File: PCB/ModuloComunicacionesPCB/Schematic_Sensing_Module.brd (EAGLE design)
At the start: 160 x 100 mm, 73 parts, among them J1 TERMINAL-TB3, J2 TERMINAL-TB3, J3 TERMINAL-TB3, J4 TERMINAL-TB3, Q1 CSM-7X-DU, Q2 MMBT2222A, SW2 1825910-6, U1 ATMEGA328P-PU, U2 LP38692MP-5.0, U3 MCP1501T-18E/SN, U4 ACS723LLCTR-05AB-T, U5 OPA320AIDBVR

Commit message: avances en placing de la pcb del transmisor
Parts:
- removed BAT_PIN: (no value), pinhead:1X02
- removed C24: (no value), rcl:C0805
- removed FTDI_PIN: (no value), pinhead:1X04
- removed J1, J2, J3, J4: TERMINAL-TB3, TERMINAL-TB001:TERMINAL-TB3
- removed Q2: MMBT2222A, MMBT2222A:SOT23
- removed R15, R16, R17, R3, R4, R5: 0.1, rcl:R1206
- removed U$2, U$7: REF3450, SOT95P280X145-6N:SOT95P280X145-6N
- removed U$3: MCP6002-E/MS, MCP6002-E_MS:SOP65P490X110-8N
- removed U$6: TERMINAL-TB2, TERMINAL-TB001:TERMINAL-TB2
- removed U2: LP38692MP-5.0, LP38692MP-5.0:SOT150P696X180-5N
- removed U4: ACS723LLCTR-05AB-T, ACS723LLCTR-05AB-T:SOIC127P600X175-8N
- removed U5: OPA320AIDBVR, OPA320AIDBVR:SOT95P280X145-5N
- added 2N2222: MMBT2222A, MMBT2222A:SOT23
- added ACS723: ACS723LLCTR-05AB-T, ACS723LLCTR-05AB-T:SOIC127P600X175-8N
- added C29, C30, C31, C32: 0.1uF, rcl:C1206
- added C33: 1nF, rcl:C1206
- added C34, C35: 2.2uF, rcl:C1206
- added IACT: (no value), TERMINAL-TB001:TERMINAL-TB2
- added JP1: (no value), pinhead:1X04/90
- added LP38692: LP38692MP-5.0, LP38692MP-5.0:SOT150P696X180-5N
- added MCP6002: MCP6002-E/MS, MCP6002-E_MS:SOP65P490X110-8N
- added OPA320: OPA320AIDBVR, OPA320AIDBVR:SOT95P280X145-5N
- added R3450, REF3450: REF3450, SOT95P280X145-6N:SOT95P280X145-6N
- added TS1, TS2, WS1, WS2: (no value), TERMINAL-TB001:TERMINAL-TB3
- C11, C12: value 22p -> 22pF; device rcl:C1206 -> rcl:C0805
- C14, C15, C20, C21: value 100n -> 100nF
- C17: value 8.2pF -> 18pF
- C2, C3: value 1uF -> cambiar por los de 10uF ceramicos de didacticas
- C22: value 0.1u -> 0.1uF
- C25, C26, C27, C28: value 0.1nF -> 0.1uF
- U$4: value INA219_BB -> INABB; device INA219_BB:INA219_BB -> INA219BB:INA219-MODULE
- moved C27 315.3 mm to (98.1, 114.0)
- moved C28 309.0 mm to (80.7, 116.0)
- moved C22 235.1 mm to (151.1, 114.0)
- moved C25 210.0 mm to (60.2, 23.8), turned to 180 degrees
- moved U$8 208.7 mm to (83.3, 59.1), turned to 270 degrees
- moved R19 205.8 mm to (60.1, 18.4), turned to 180 degrees
- moved LED4 199.4 mm to (115.7, 74.0), turned to 90 degrees
- moved C26 196.9 mm to (46.2, 17.6), turned to 270 degrees
- moved LED3 195.6 mm to (116.1, 66.9), turned to 270 degrees
- moved R1 192.7 mm to (90.5, 38.5), turned to 180 degrees
- moved R12 191.1 mm to (98.1, 106.3)
- moved R7 189.3 mm to (107.7, 67.0), turned to 180 degrees
- moved SW2 187.5 mm to (115.8, 57.7), turned to 90 degrees
- moved R18 186.2 mm to (41.4, 17.6), turned to 270 degrees
- moved C23 170.4 mm to (66.0, 38.5)
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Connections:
- removed net +5V: U$1.IN+
- removed net A0: U1.23
- removed net A1: U1.24
- removed net A2: U1.25
- removed net A3: U1.26
- removed net N$1: R3.2, U$2.1
- removed net N$10: U$6.1, U4.1, U4.2
- removed net N$11: U$6.2, U4.3, U4.4
- removed net N$12: R11.2, U4.7
- removed net N$13: C9.1, R12.2, U5.3
- removed net N$15: C10.1, R13.1, U5.1, U5.4
- removed net N$18: R16.2, U$7.6
- removed net N$19: R17.2, U$7.5
- removed net N$20: R15.2, U$7.1
- removed net N$24: C25.1, R19.1, U$3.3
- removed net N$25: C26.1, R18.1, U$3.5
- removed net N$5: R4.2, U$2.6
- removed net N$6: R5.2, U$2.5
- removed net N$8: R10.1, U4.6
- removed net VOUT-: U$1.VOUT-
- new net BWSEL: ACS723.6, R10.1
- new net IP+: ACS723.1, ACS723.2, IACT.1
- new net IP-: ACS723.3, ACS723.4, IACT.2
- new net VIN+: C9.1, OPA320.3, R12.2
- new net VIN-: C10.1, OPA320.1, OPA320.4, R13.1
- new net VO: ACS723.7, C33.1, R11.2
- net B+INA: now also U$4.6
- net B-INA: now also U$4.5; no longer BAT_PIN.1
- net BATL: now also U1.13; no longer U1.11
- net DATAT1: now also TS1.2, U1.14; no longer J3.2
- net DATAT2: now also TS2.2, U1.15; no longer J4.2
- net DATAW1: now also C25.1, MCP6002.3, R19.1, WS1.3; no longer J1.3
- net DATAW2: now also C26.1, MCP6002.5, R18.1, WS2.3; no longer J2.3
- net DTR: now also JP1.4; no longer FTDI_PIN.4
- net GND: now also ACS723.5, C29.2, C30.2, C31.2, C32.2, C33.2, C34.1, C35.2, JP1.1, LP38692.5, MCP6002.4, OPA320.2, R3450.1, R3450.2, REF3450.1, REF3450.2, TS1.3, TS2.3, U$1.VOUT-, U$4.2, U$8.DIO0, U$8.DIO1, U$8.DIO2, U$8.DIO3, U$8.DIO4, U1.25, U1.26, U1.6, WS1.1, WS2.1; no longer BAT_PIN.2, C24.2, FTDI_PIN.1, J1.1, J2.1, J3.3, J4.3, R15.1, R3.1, U$2.2, U$3.4, U$7.2, U2.5, U4.5, U5.2
- net N$2: now also 2N2222.1; no longer Q2.1
- net OSC+: now also C12.1; no longer C11.1
- net OSC-: now also C11.1; no longer C12.1
- net RX0: now also JP1.3; no longer FTDI_PIN.3
- net RX1: now also U$8.TX
- net SCL: now also U$4.3
- net SDA: now also U$4.4
- net TX0: now also JP1.2; no longer FTDI_PIN.2
- net TX1: now also U$8.RX
- net VACS: now also ACS723.8, REF3450.5, REF3450.6; no longer R16.1, R17.1, U4.8
- net VDD33: now also C29.1, U$4.1; no longer C17.1, C24.1
- net VLP5: now also C30.1, C31.1, C32.1, C34.2, LP38692.3, MCP6002.8, TS1.1, TS2.1, U1.21, WS1.2, WS2.2; no longer J1.2, J2.2, J3.1, J4.1, U$3.8, U2.3
- net VOREG: now also 2N2222.2, R3450.3, R3450.4, REF3450.3, REF3450.4; no longer Q2.2, U$2.3, U$2.4, U$7.3, U$7.4
- net VOUT+: now also C17.1, C35.1
- net VOW1: now also MCP6002.1, MCP6002.2, U1.23; no longer U$3.1, U$3.2
- net VOW2: now also MCP6002.6, MCP6002.7, U1.24; no longer U$3.6, U$3.7
- net VREF5: now also OPA320.5, R3450.5, R3450.6; no longer R4.1, R5.1, U5.5
- net VSUPPLY: now also 2N2222.3, LP38692.1, LP38692.4; no longer Q2.3, U2.1, U2.4

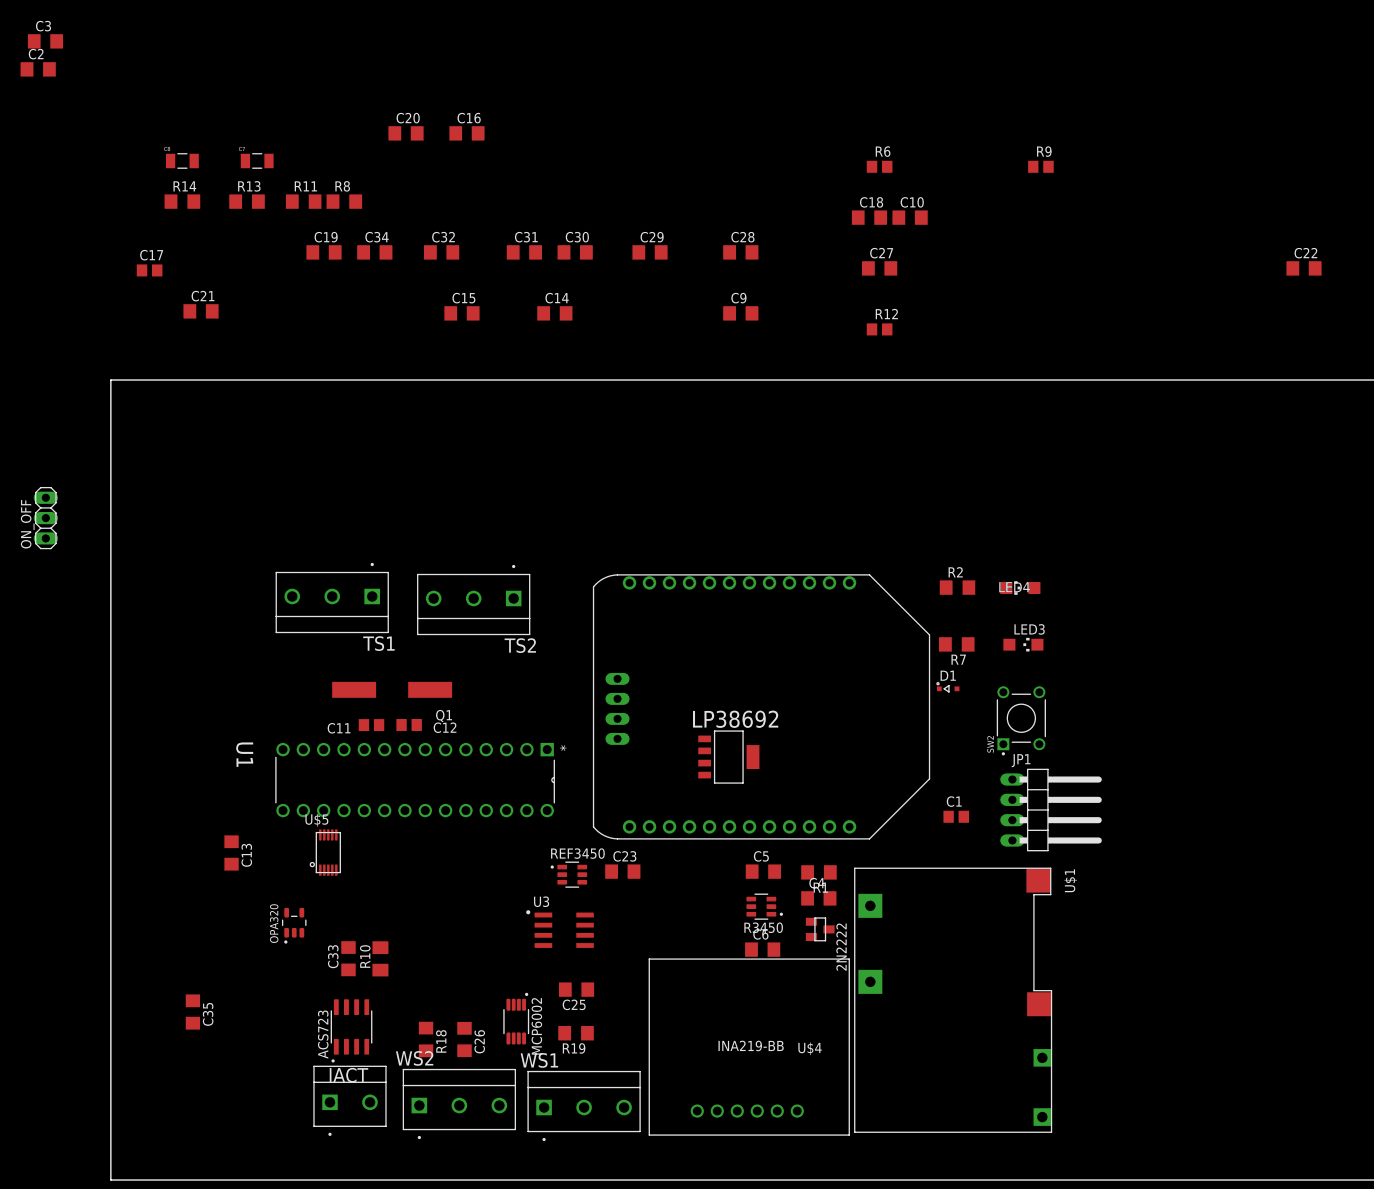
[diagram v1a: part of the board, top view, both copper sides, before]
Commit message: placing almost done
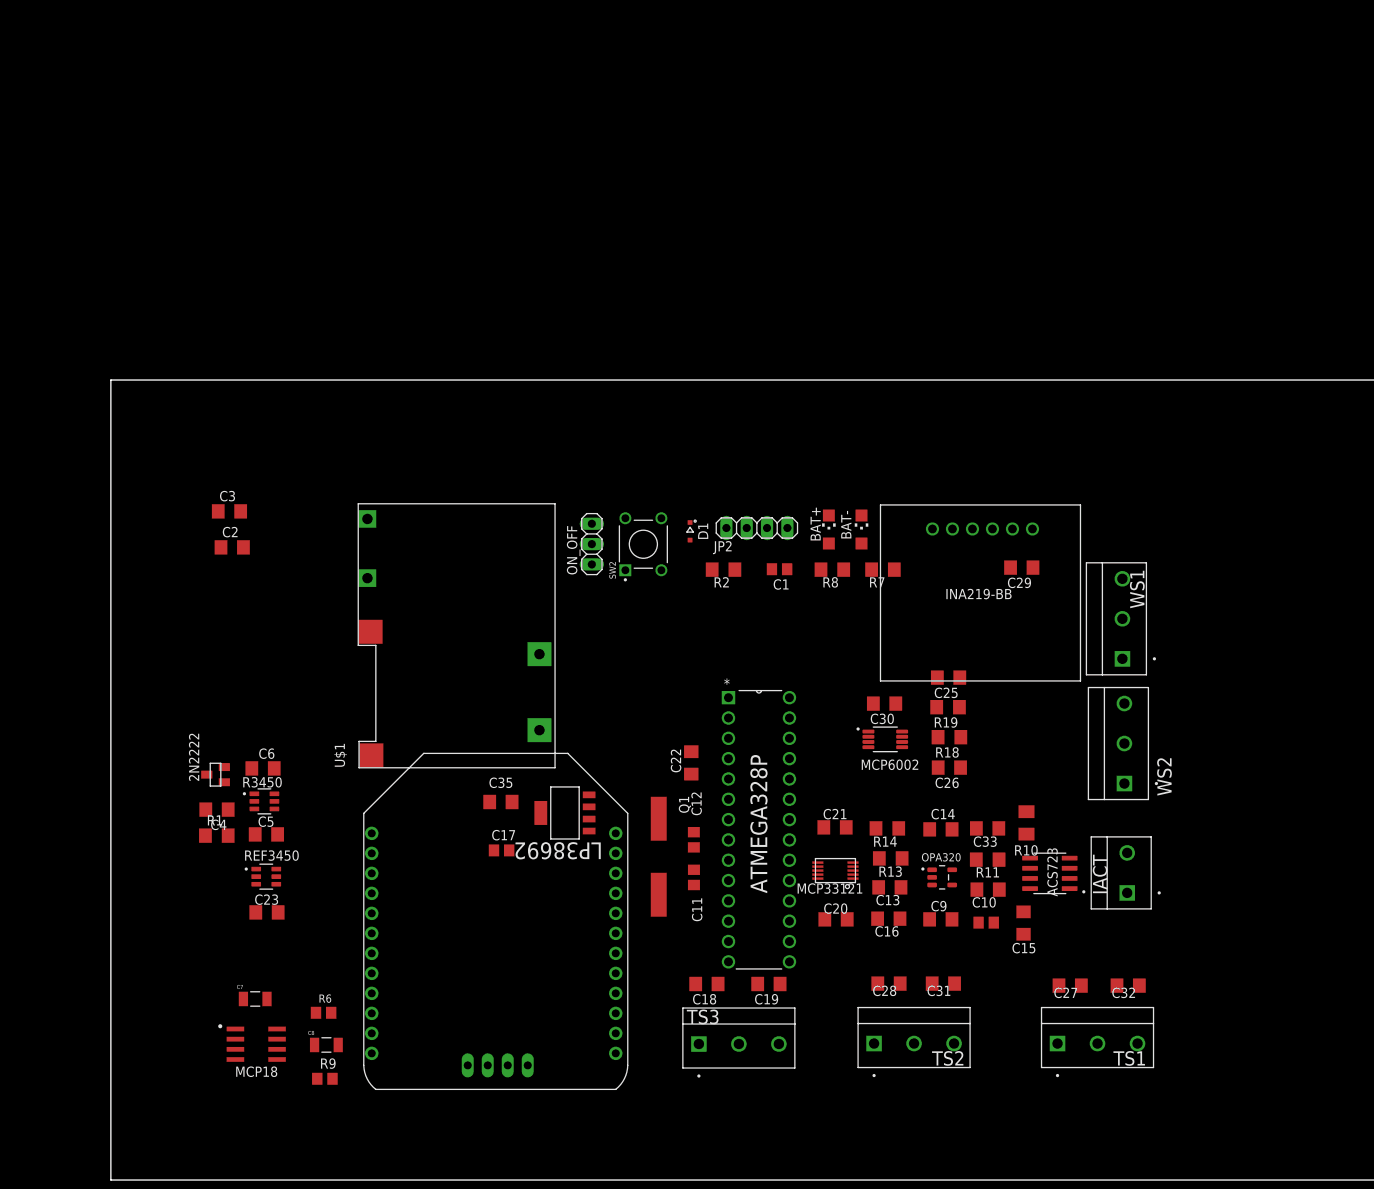
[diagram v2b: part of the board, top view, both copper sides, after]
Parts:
- removed C34: 2.2uF, rcl:C1206
- removed JP1: (no value), pinhead:1X04/90
- removed LED3, LED4: (no value), led:CHIPLED_1206
- removed U$4: INABB, INA219BB:INA219-MODULE
- removed U$5: MCP33121, mcp33121:MSOP10
- removed U1: ATMEGA328P-PU, Atmel_By_element14_Batch_1-00:DIP254P762X457-28
- removed U3: MCP1501T-18E/SN, MCP1501T-18E_SN:SOIC127P600X175-8N
- added ATMEGA328P: ATMEGA328P-PU, Atmel_By_element14_Batch_1-00:DIP254P762X457-28
- added BAT+, BAT-: (no value), led:CHIPLED_1206
- added INA219: INABB, INA219BB:INA219-MODULE
- added JP2: (no value), pinhead:1X04
- added MCP18: MCP1501T-18E/SN, MCP1501T-18E_SN:SOIC127P600X175-8N
- added MCP33121: MCP33121, mcp33121:MSOP10
- added TS3: (no value), TERMINAL-TB001:TERMINAL-TB3
- C18: value 1uF -> 0.1uF
- C19: value 10uF -> 0.1uF
- moved R9 144.9 mm to (28.8, 12.7)
- moved R6 126.5 mm to (28.6, 20.9)
- moved C32 125.6 mm to (129.2, 24.3), turned to 180 degrees
- moved R11 118.6 mm to (111.6, 40.0)
- moved R14 117.9 mm to (99.1, 44.0), turned to 180 degrees
- moved R13 115.0 mm to (99.5, 40.2), turned to 180 degrees
- moved C20 112.0 mm to (92.6, 32.6), turned to 180 degrees
- moved C8 112.0 mm to (28.9, 16.9)
- moved C16 111.4 mm to (99.2, 32.7)
- moved C19 107.0 mm to (84.2, 24.5), turned to 180 degrees
- moved C31 105.3 mm to (106.1, 24.6), turned to 180 degrees
- moved C7 104.8 mm to (20.0, 22.6)
- moved C15 103.6 mm to (116.1, 32.1), turned to 270 degrees
- moved C21 102.2 mm to (92.5, 44.1)
- moved IACT 101.3 mm to (129.0, 38.4), turned to 90 degrees
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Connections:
- removed net N$16: C13.2, R13.2, U$5.3
- removed net N$17: C13.1, R14.2, U$5.4
- removed net N$7: R6.2, R9.2, U3.7, U3.8
- new net DATAT3: ATMEGA328P.13, C18.1, TS3.2
- new net IN+: C13.2, MCP33121.3, R13.2
- new net IN-: C13.1, MCP33121.4, R14.2
- new net VOMCP18: MCP18.7, MCP18.8, R6.2, R9.2
- net AMISO: now also ATMEGA328P.18, MCP33121.7; no longer U$5.7, U1.18
- net AMOSI: now also ATMEGA328P.17, MCP33121.9; no longer U$5.9, U1.17
- net ASCK: now also ATMEGA328P.19, MCP33121.8; no longer U$5.8, U1.19
- net ASS: now also ATMEGA328P.16, MCP33121.6; no longer U$5.6, U1.16
- net B+INA: now also INA219.6; no longer U$4.6
- net B-INA: now also INA219.5; no longer U$4.5
- net BATH: now also ATMEGA328P.11; no longer U1.12
- net BATL: now also ATMEGA328P.12; no longer U1.13
- net DATAT1: now also ATMEGA328P.14; no longer U1.14
- net DATAT2: now also ATMEGA328P.15; no longer U1.15
- net DTR: now also JP2.4; no longer JP1.4
- net GND: now also ATMEGA328P.22, ATMEGA328P.25, ATMEGA328P.26, ATMEGA328P.6, ATMEGA328P.8, BAT+.C, BAT-.C, C19.2, INA219.2, JP2.1, MCP18.2, MCP18.4, MCP18.5, MCP18.6, MCP33121.5, TS1.1, TS2.1, TS3.1; no longer C19.1, C34.1, JP1.1, LED3.C, LED4.C, TS1.3, TS2.3, U$4.2, U$5.5, U1.22, U1.25, U1.26, U1.6, U1.8, U3.2, U3.4, U3.5, U3.6
- net N$3: now also BAT-.A; no longer LED3.A
- net N$4: now also BAT+.A; no longer LED4.A
- net OSC+: now also ATMEGA328P.9; no longer U1.9
- net OSC-: now also ATMEGA328P.10; no longer U1.10
- net RST: now also ATMEGA328P.1; no longer U1.1
- net RX0: now also ATMEGA328P.2, JP2.3; no longer JP1.3, U1.2
- net RX1: now also ATMEGA328P.4; no longer U1.4
- net SCL: now also ATMEGA328P.28, INA219.3; no longer U$4.3, U1.28
- net SDA: now also ATMEGA328P.27, INA219.4; no longer U$4.4, U1.27
- net TX0: now also ATMEGA328P.3, JP2.2; no longer JP1.2, U1.3
- net TX1: now also ATMEGA328P.5; no longer U1.5
- net VDD33: now also INA219.1; no longer U$4.1
- net VLP5: now also ATMEGA328P.20, ATMEGA328P.21, ATMEGA328P.7, C19.1, MCP33121.10, TS1.3, TS2.3, TS3.3; no longer C19.2, C34.2, TS1.1, TS2.1, U$5.10, U1.20, U1.21, U1.7
- net VOW1: now also ATMEGA328P.23; no longer U1.23
- net VOW2: now also ATMEGA328P.24; no longer U1.24
- net VREF18: now also MCP33121.2; no longer U$5.2
- net VREF5: now also MCP18.1, MCP18.3, MCP33121.1; no longer C18.1, U$5.1, U3.1, U3.3

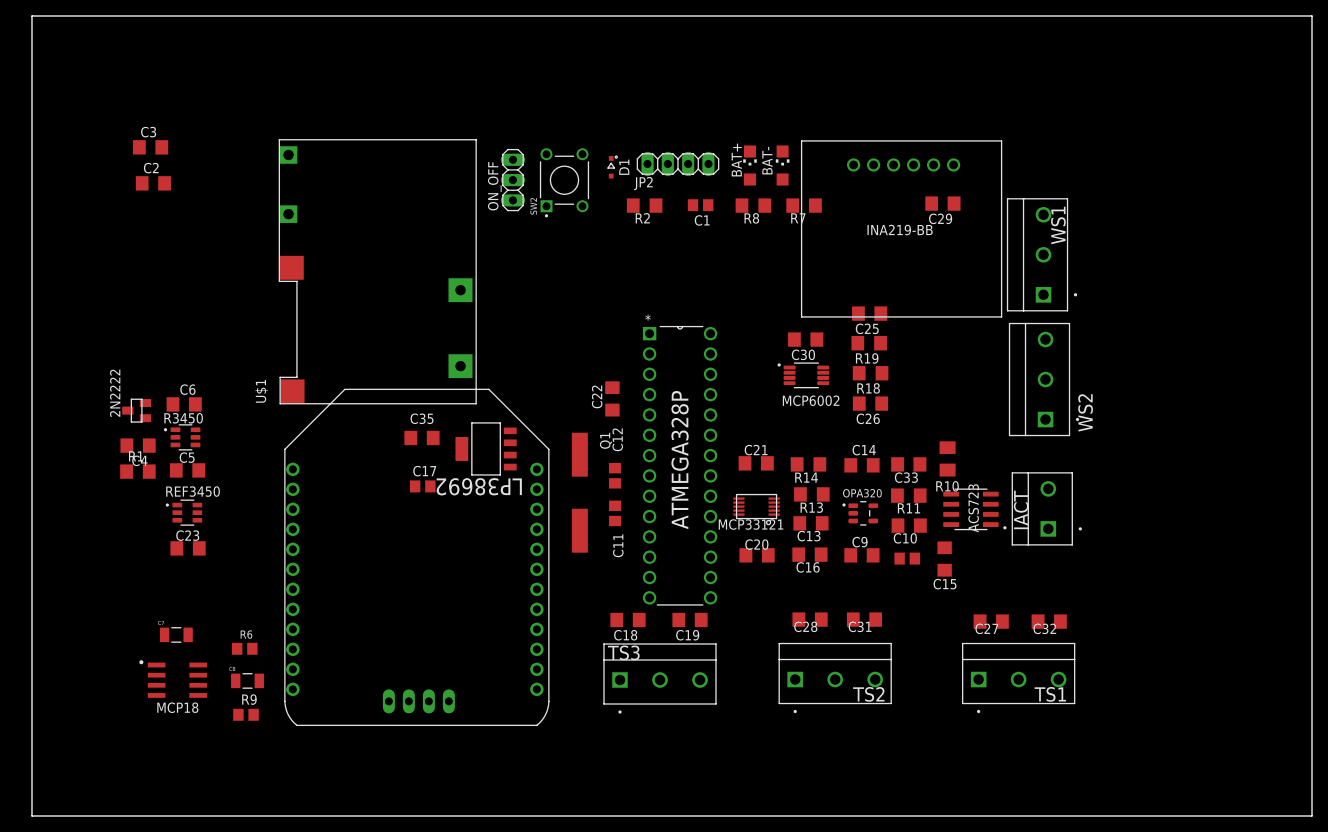
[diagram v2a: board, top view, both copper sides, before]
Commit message: Finished Placing-Give a review
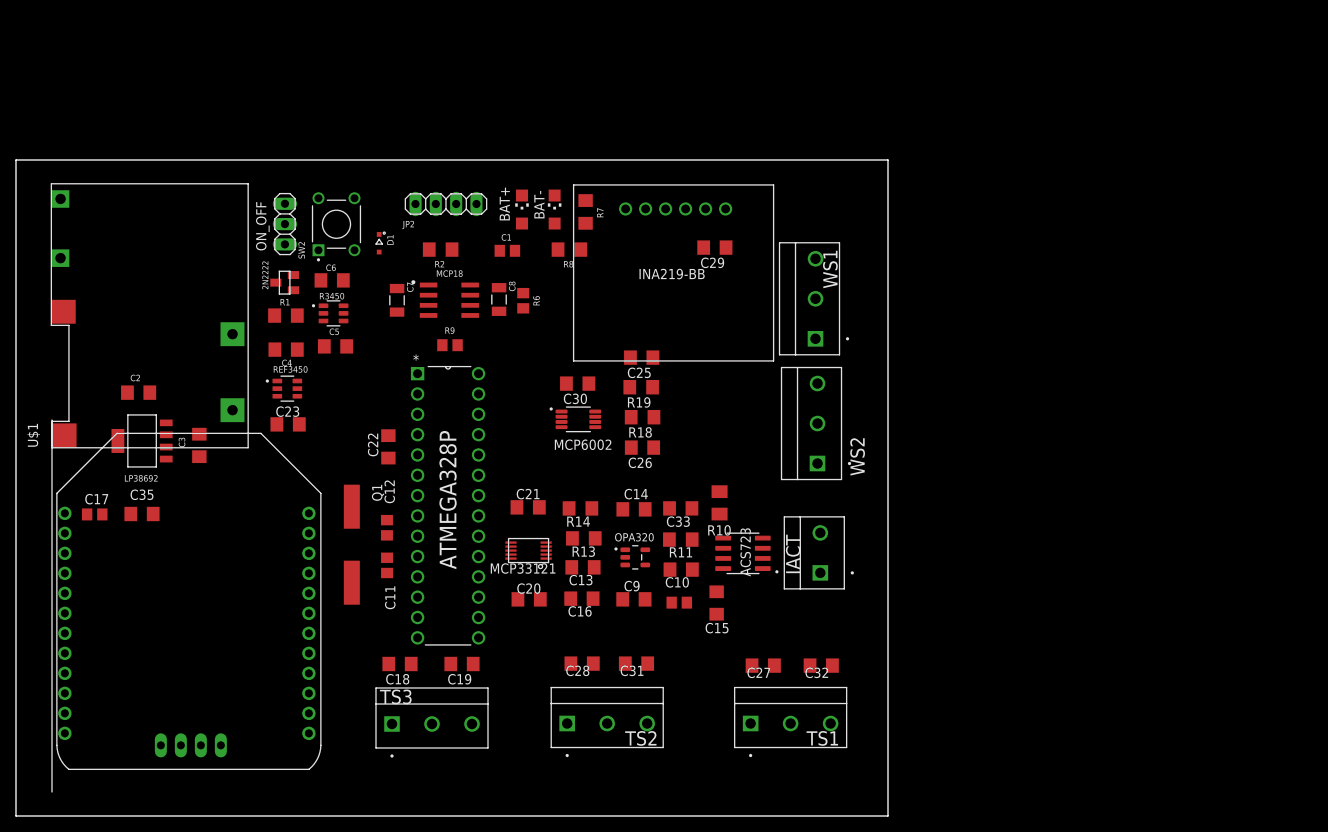
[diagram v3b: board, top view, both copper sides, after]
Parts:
- C2, C3: value cambiar por los de 10uF ceramicos de didacticas -> 10uF
- C23, C6: value 1u -> 10u
- moved MCP18 58.4 mm to (54.2, 64.5)
- moved C8 57.1 mm to (60.4, 64.6), turned to 270 degrees
- moved R6 55.7 mm to (63.4, 64.4), turned to 270 degrees
- moved R9 52.8 mm to (54.2, 58.9), turned to 180 degrees
- moved C7 50.1 mm to (47.6, 64.5), turned to 270 degrees
- moved LP38692 43.0 mm to (15.8, 46.9)
- moved C17 41.1 mm to (9.84, 37.7)
- moved C3 37.8 mm to (22.9, 46.3), turned to 90 degrees
- moved C35 36.3 mm to (15.8, 37.8)
- moved D1 30.5 mm to (45.4, 71.6)
- moved JP2 29.4 mm to (53.8, 76.5)
- moved ATMEGA328P 29.4 mm to (57.8, 22.3)
- moved C12 29.2 mm to (46.4, 36.0)
- moved Q1 29.2 mm to (42.0, 33.9)
- moved C11 29.2 mm to (46.4, 31.3)
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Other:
- board size 160 x 100 mm -> 109 x 82 mm
